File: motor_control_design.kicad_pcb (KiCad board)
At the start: 2 copper layers, 57.1 x 57.2 mm, 102 parts, among them J1 TYPE-C-31-M-12, J10 5V, J2 SWD, J3 VBAT, J4 GND, J5 FC_M/P, J6 Conn_01x06, J7 Conn_01x04_Pin, J8 Conn_01x06, J9 GND, Q1 RF1S9540SM, Q10 2N7002, Q11 2N7002, Q12 2N7002, Q13 2N7002, Q14 RF1S9540SM, Q15 IRLZ44NS, Q16 2N7002, Q2 RF1S9540SM, Q3 IRLZ44NS, Q4 2N7002, Q5 2N7002, Q6 RF1S9540SM, Q7 IRLZ44NS, Q8 2N7002, Q9 IRLZ44NS, U1 STM32F401CCU6, U2 LT1962-3.3, U3 LTC4365DDB, U4 TPS563200, Y1 16MHz

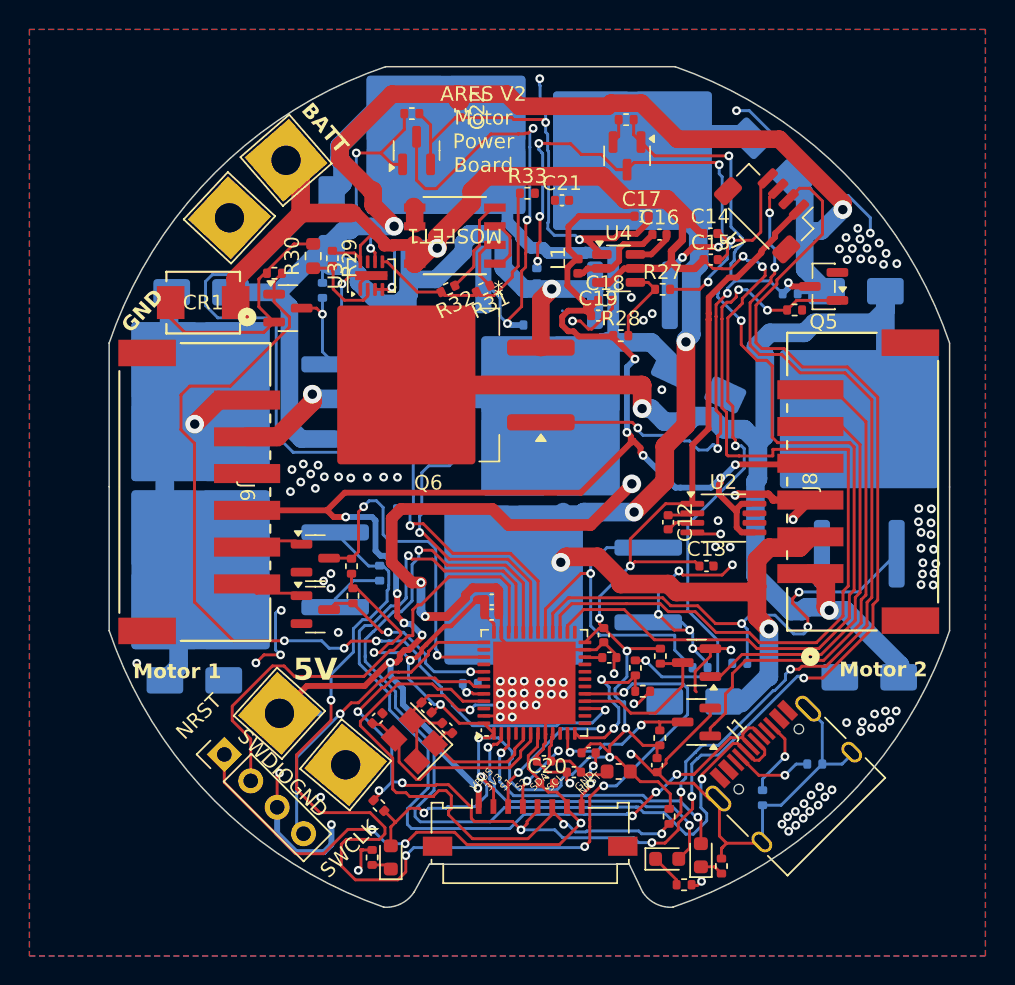
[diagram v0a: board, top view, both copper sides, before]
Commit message: original placement
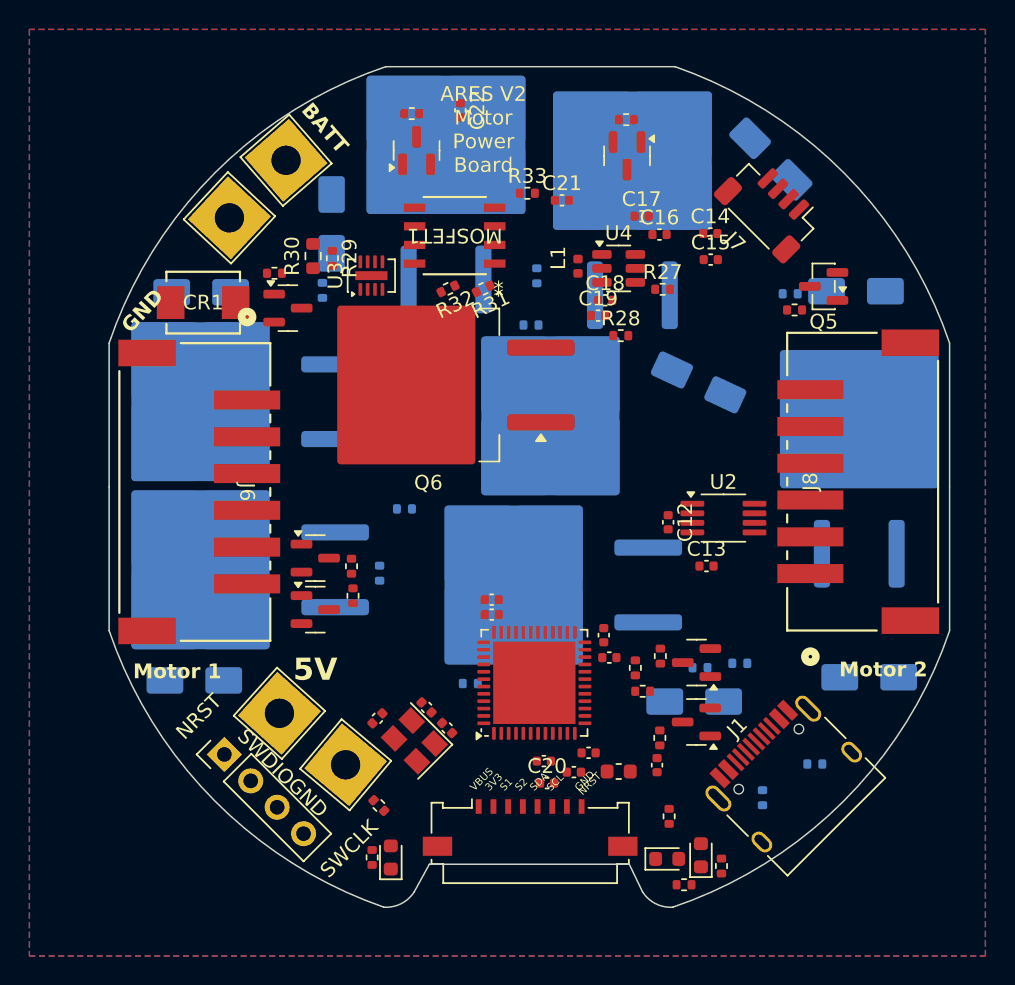
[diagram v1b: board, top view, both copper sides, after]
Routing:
- net GND: track 258.7 -> 0.00 mm, vias 128 -> 0
- net +3.3V: track 128.6 -> 0.00 mm, vias 11 -> 0
- net VMOTOR: track 127.2 -> 0.00 mm, vias 4 -> 0
- net +5V: track 118.7 -> 0.00 mm, vias 11 -> 0
- net +BATT: track 115.9 -> 0.00 mm, vias 6 -> 0
- net /SDA: track 103.0 -> 0.00 mm, vias 7 -> 0
- net /SCL: track 97.9 -> 0.00 mm, vias 6 -> 0
- net /M2A: track 80.3 -> 0.00 mm, vias 2 -> 0
- net /M1Q2: track 74.8 -> 0.00 mm, vias 5 -> 0
- net /M1Q3: track 70.5 -> 0.00 mm, vias 2 -> 0
- net /M2B: track 70.2 -> 0.00 mm, vias 4 -> 0
- net /M2Q3: track 69.9 -> 0.00 mm, vias 2 -> 0
- net /USB_D-: track 65.7 -> 0.00 mm, vias 2 -> 0
- net /USB_D+: track 63.4 -> 0.00 mm, vias 4 -> 0
- net /M1Q1: track 62.4 -> 0.00 mm, vias 4 -> 0
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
